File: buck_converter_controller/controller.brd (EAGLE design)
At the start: 83.8 x 88.6 mm, 17 parts

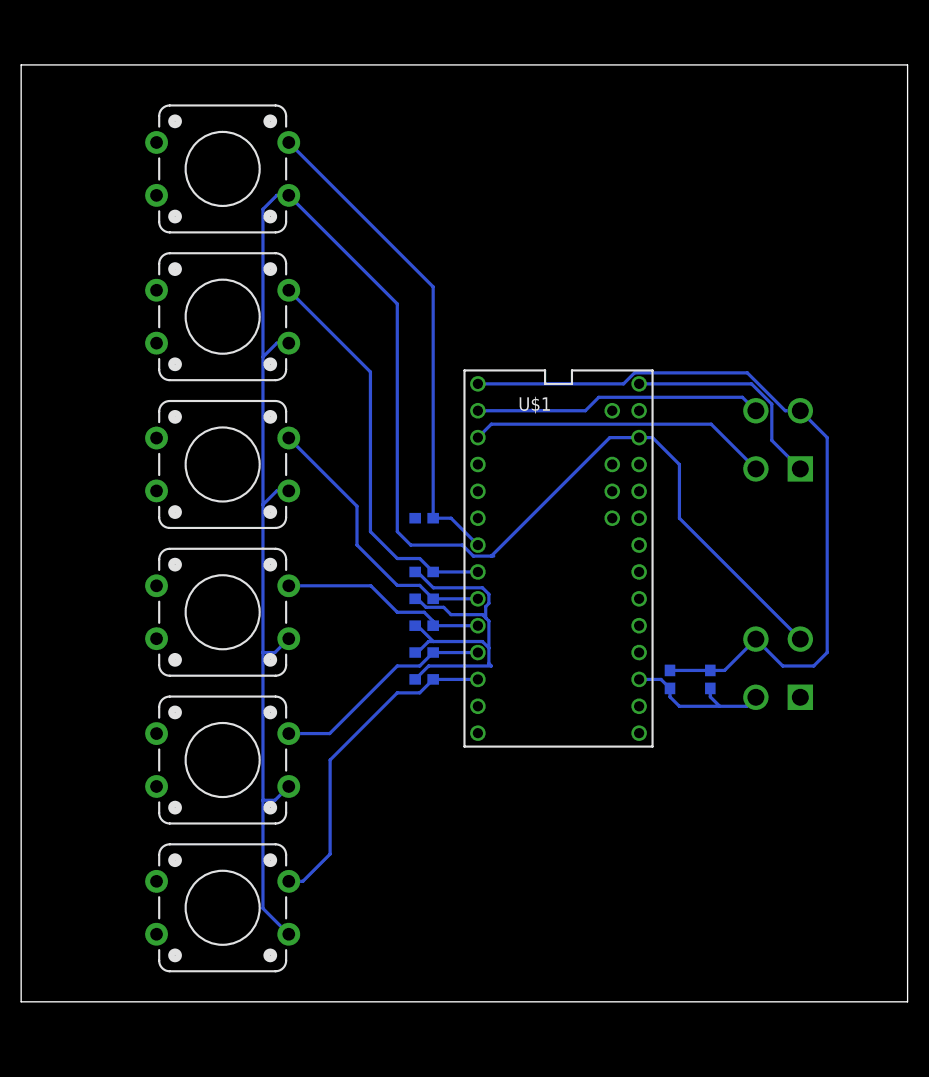
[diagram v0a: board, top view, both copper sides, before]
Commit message: Update controller.brd
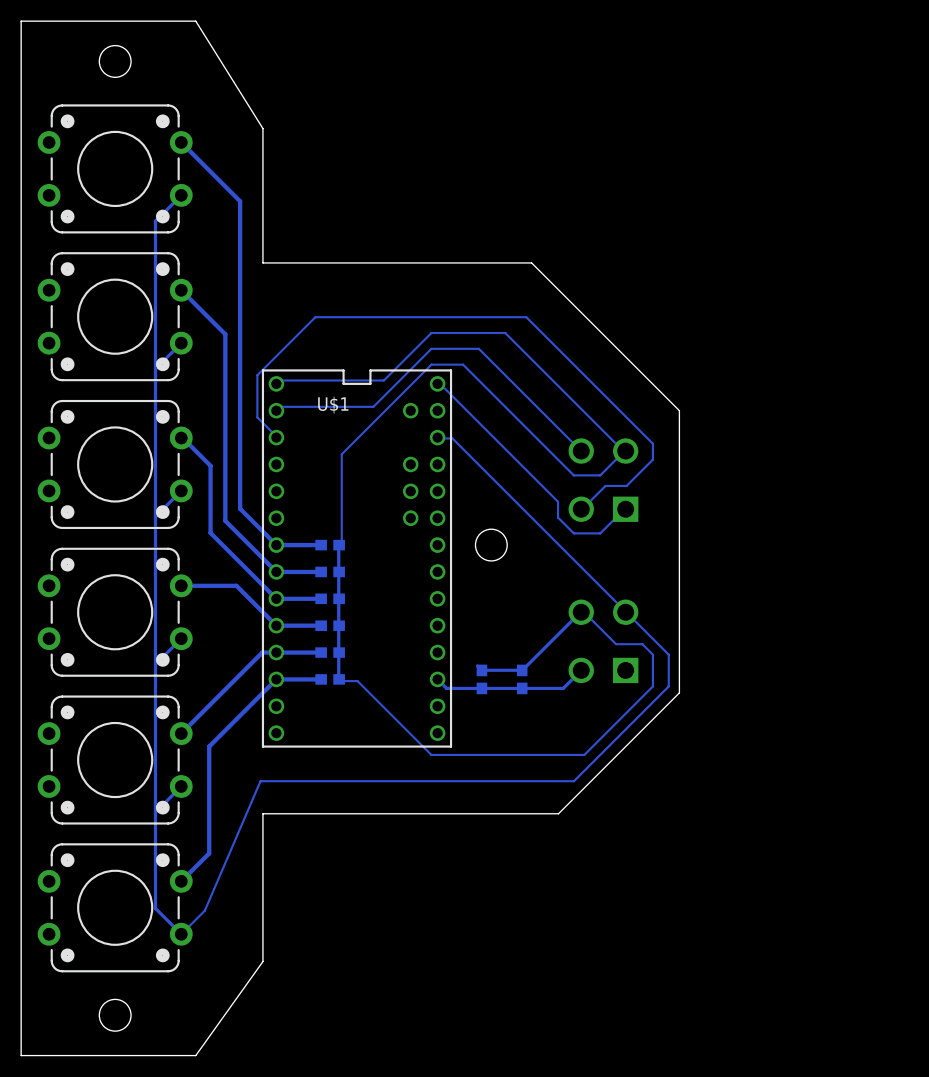
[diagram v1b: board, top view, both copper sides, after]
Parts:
- moved U$1 19.0 mm to (31.8, 47.0)
- moved C39 17.8 mm to (43.6, 35.6)
- moved R26 17.8 mm to (47.4, 35.6)
- moved SERIAL1 16.9 mm to (57.1, 57.1)
- moved U$17 16.7 mm to (57.1, 41.9)
- moved S1 10.2 mm to (8.89, 83.8)
- moved S2 10.2 mm to (8.89, 69.8)
- moved S3 10.2 mm to (8.89, 55.9)
- moved S4 10.2 mm to (8.89, 41.9)
- moved S5 10.2 mm to (8.89, 27.9)
- moved S6 10.2 mm to (8.89, 14.0)
- moved R1 9.25 mm to (29.2, 48.3), turned to 180 degrees
- moved R2 8.89 mm to (29.2, 45.7), turned to 180 degrees
- moved R3 8.89 mm to (29.2, 43.2), turned to 180 degrees
- moved R4 8.89 mm to (29.2, 40.6), turned to 180 degrees
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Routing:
- net GND: track 114.1 -> 156.3 mm
- net TX: track 28.6 -> 61.4 mm
- net RX: track 27.3 -> 35.3 mm
- net BUT4: track 19.7 -> 14.8 mm
- net VIN: track 20.6 -> 25.4 mm
- net BUT5: track 21.1 -> 16.4 mm
- net BUT6: track 31.0 -> 27.0 mm
- net BUT2: track 37.8 -> 34.6 mm
- net BUT3: track 26.3 -> 23.2 mm
- net 3V: track 175.3 -> 177.8 mm
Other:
- board size 83.8 x 88.6 mm -> 62.2 x 97.8 mm
